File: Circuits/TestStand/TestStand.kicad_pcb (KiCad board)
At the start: 2 copper layers, 72.5 x 95 mm, 53 parts, among them J1 Screw_Terminal_01x07, J10 Screw_Terminal_01x03, J11 Screw_Terminal_01x03, J12 Screw_Terminal_01x03, J13 Screw_Terminal_01x03, J2 Screw_Terminal_01x07, J3 Screw_Terminal_01x07, J4 Screw_Terminal_01x03, J5 Screw_Terminal_01x03, J6 Screw_Terminal_01x03, J7 Screw_Terminal_01x03, J8 Screw_Terminal_01x03, J9 Screw_Terminal_01x03, Q1 MMBT4403-7-F, Q2 MMBT4403-7-F, Q3 MMBT4403-7-F, U1 HX711, U2 HX711, U3 HX711, U4 Teensy4.1

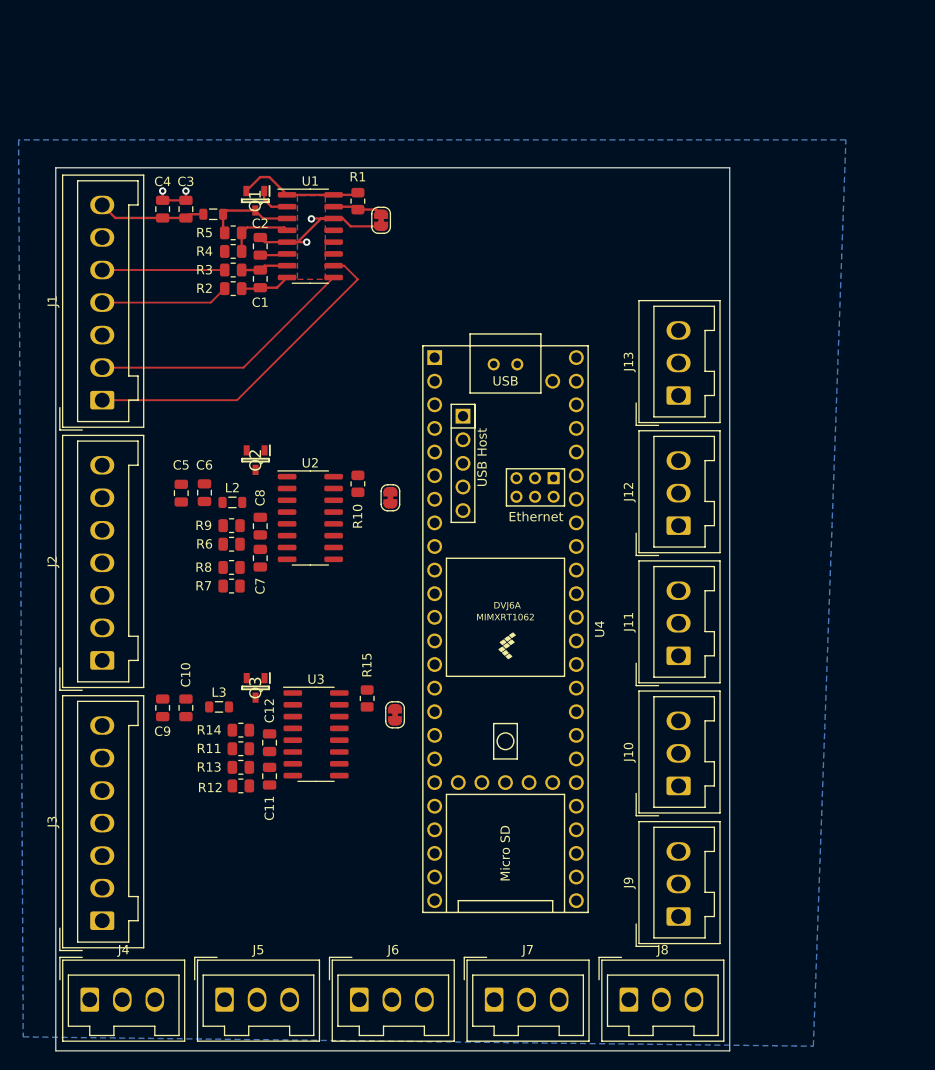
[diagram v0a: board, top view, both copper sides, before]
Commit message: did some traces
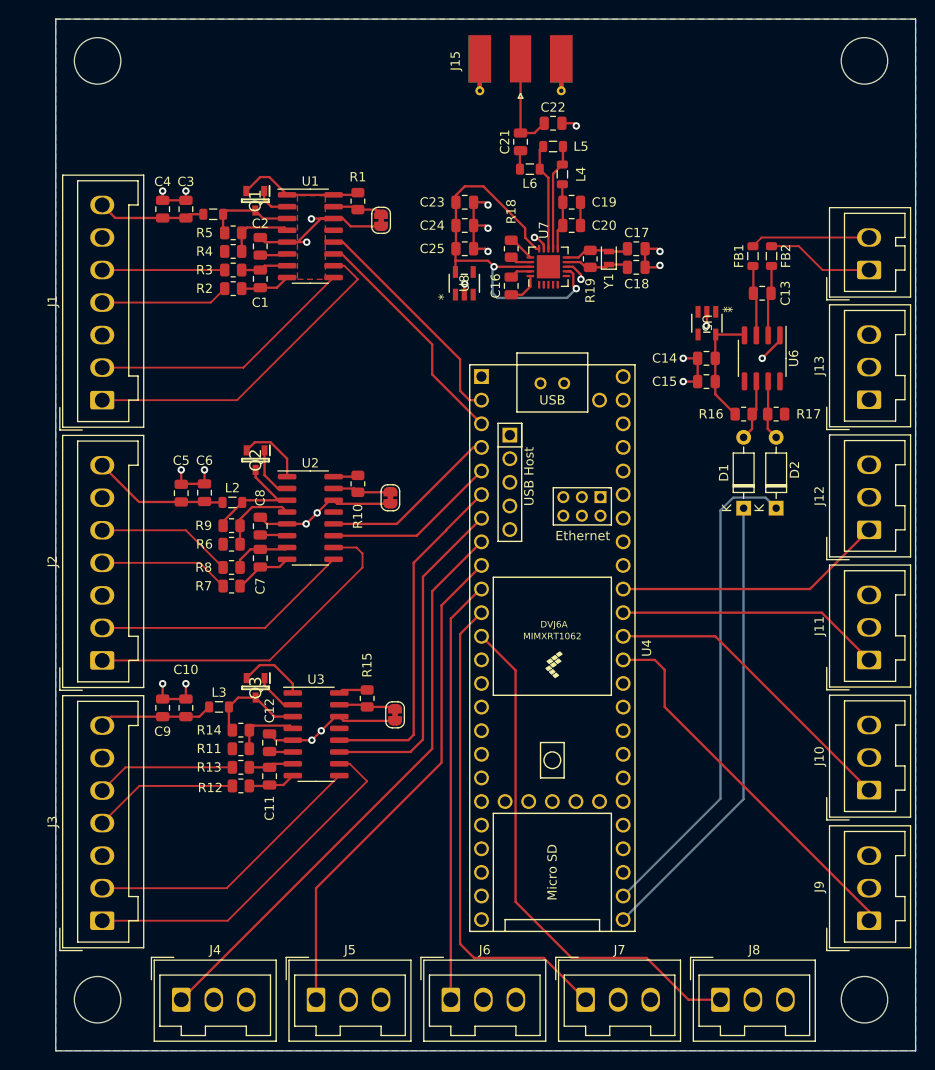
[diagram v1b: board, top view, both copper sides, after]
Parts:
- added C13: 0.01uF, Capacitor_SMD:C_0805_2012Metric, F.Cu at (98.5, 92.5)
- added C14: 10uF, Capacitor_SMD:C_0805_2012Metric, F.Cu at (92.5, 99.5)
- added C15: 10uF, Capacitor_SMD:C_0805_2012Metric, F.Cu at (92.5, 102.0)
- added C16: 33nF, Capacitor_SMD:C_0805_2012Metric, F.Cu at (71.5, 91.7)
- added C17: 22pF, Capacitor_SMD:C_0805_2012Metric, F.Cu at (85.0, 87.7)
- added C18: 22pF, Capacitor_SMD:C_0805_2012Metric, F.Cu at (85.0, 89.7)
- added C19: 2.2uF, Capacitor_SMD:C_0805_2012Metric, F.Cu at (78.0, 82.7)
- added C20: 4.7pF, Capacitor_SMD:C_0805_2012Metric, F.Cu at (78.0, 85.2)
- added C21: 1.5pF, Capacitor_SMD:C_0805_2012Metric, F.Cu at (72.5, 76.2)
- added C22: 1pF, Capacitor_SMD:C_0805_2012Metric, F.Cu at (76.0, 74.2)
- added C23: 10uF, Capacitor_SMD:C_0805_2012Metric, F.Cu at (66.5, 82.7)
- added C24: 10nF, Capacitor_SMD:C_0805_2012Metric, F.Cu at (66.5, 85.2)
- added C25: 1nF, Capacitor_SMD:C_0805_2012Metric, F.Cu at (66.5, 87.7)
- added D1: 1N4148, Diode_THT:D_DO-35_SOD27_P7.62mm_Horizontal, F.Cu at (96.5, 115.6)
- added D2: 1N4148, Diode_THT:D_DO-35_SOD27_P7.62mm_Horizontal, F.Cu at (100.0, 115.6)
- added FB1: FerriteBead, Inductor_SMD:L_0805_2012Metric, F.Cu at (97.5, 88.5)
- added FB2: FerriteBead, Inductor_SMD:L_0805_2012Metric, F.Cu at (99.5, 88.5)
- added J14: Screw_Terminal_01x02, Connector_Wago:Wago_734-132_1x02_P3.50mm_Vertical, F.Cu at (110.0, 90.0)
- added J15: Conn_Coaxial, Connector_Coaxial:SMA_Molex_73251-1153_EdgeMount_Horizontal, F.Cu at (72.5, 69.0)
- added L4: 2.7nH, Inductor_SMD:L_0805_2012Metric, F.Cu at (77.0, 79.7)
- added L5: 8.2nH, Inductor_SMD:L_0805_2012Metric, F.Cu at (76.0, 76.7)
- added L6: 3.9nH, Inductor_SMD:L_0805_2012Metric, F.Cu at (73.5, 79.1)
- added R16: 10k, Resistor_SMD:R_0805_2012Metric, F.Cu at (96.5, 105.5)
- added R17: 10k, Resistor_SMD:R_0805_2012Metric, F.Cu at (100.0, 105.5)
- added R18: 22k, Resistor_SMD:R_0805_2012Metric, F.Cu at (71.5, 87.7)
- added R19: 1M, Resistor_SMD:R_0805_2012Metric, F.Cu at (80.0, 88.8)
- added U5: LP2980IM5X-3.3/NOPB, Library:MF05A_TEX, F.Cu at (92.5, 95.7)
- added U6: MAX31855KASA, Package_SO:SOIC-8_3.9x4.9mm_P1.27mm, F.Cu at (98.5, 99.5)
- added U7: NRF24L01, Package_DFN_QFN:QFN-20-1EP_4x4mm_P0.5mm_EP2.5x2.5mm, F.Cu at (75.5, 89.6)
- added U8: LP2980IM5X-3.3/NOPB, Library:MF05A_TEX, F.Cu at (66.5, 91.4)
- added Y1: 16Mhz, Crystal:Crystal_SMD_2012-2Pin_2.0x1.2mm, F.Cu at (82.0, 88.7)
- moved J10 20.5 mm to (110.0, 145.9)
- moved J11 20.5 mm to (110.0, 131.9)
- moved J12 20.5 mm to (110.0, 118.0)
- moved J13 20.5 mm to (110.0, 104.0)
- moved J9 20.5 mm to (110.0, 160.0)
- moved J4 9.84 mm to (36.0, 168.5)
- moved J5 9.84 mm to (50.5, 168.5)
- moved J6 9.84 mm to (65.0, 168.5)
- moved J7 9.84 mm to (79.5, 168.5)
- moved J8 9.84 mm to (94.0, 168.5)
- moved U4 5.44 mm to (75.9, 130.7)
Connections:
- U4 pad 18: unconnected-(U4-26_A12_MOSI1-Pad18) -> /rMOSI
- U4 pad 19: unconnected-(U4-27_A13_SCK1-Pad19) -> /rSCK
- U4 pad 20: unconnected-(U4-28_RX7-Pad20) -> /rCE
- U4 pad 21: unconnected-(U4-29_TX7-Pad21) -> /rIRQ
- U4 pad 25: unconnected-(U4-33_MCLK2-Pad25) -> /tcCS
- U4 pad 26: unconnected-(U4-34_RX8-Pad26) -> /tcSO
- U4 pad 27: unconnected-(U4-35_TX8-Pad27) -> /tcSCK
- U4 pad 30: unconnected-(U4-38_CS1_IN1-Pad30) -> /rCSN
- U4 pad 31: unconnected-(U4-39_MISO1_OUT1A-Pad31) -> /rMISO
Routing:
- net GND: track 23.6 -> 106.7 mm, vias 4 -> 25
- net /PWM0: track 0.00 -> 62.6 mm
- net /PWM4: track 0.00 -> 56.5 mm
- net /PWM1: track 0.00 -> 54.1 mm
- net /tcSO: track 0.00 -> 52.8 mm
- net /PWM3: track 0.00 -> 52.6 mm
- net /tcCS: track 0.00 -> 49.6 mm
- net /PWM2: track 0.00 -> 45.6 mm
- net /+3VRF: track 0.00 -> 44.4 mm, vias 0 -> 2
- net /PT0: track 0.00 -> 41.0 mm
- net /B2+: track 0.00 -> 38.5 mm
- net /DAT2: track 0.00 -> 37.1 mm
- net /B1+: track 0.00 -> 37.0 mm
- net /SCK2: track 0.00 -> 36.0 mm
- net /PT1: track 0.00 -> 33.3 mm
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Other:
- board size 72.5 x 95 mm -> 92.5 x 111 mm
